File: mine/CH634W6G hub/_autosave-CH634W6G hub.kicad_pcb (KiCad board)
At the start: 2 copper layers, 5 parts, among them U1 CH634W6G, U2 *, U3 CH211D

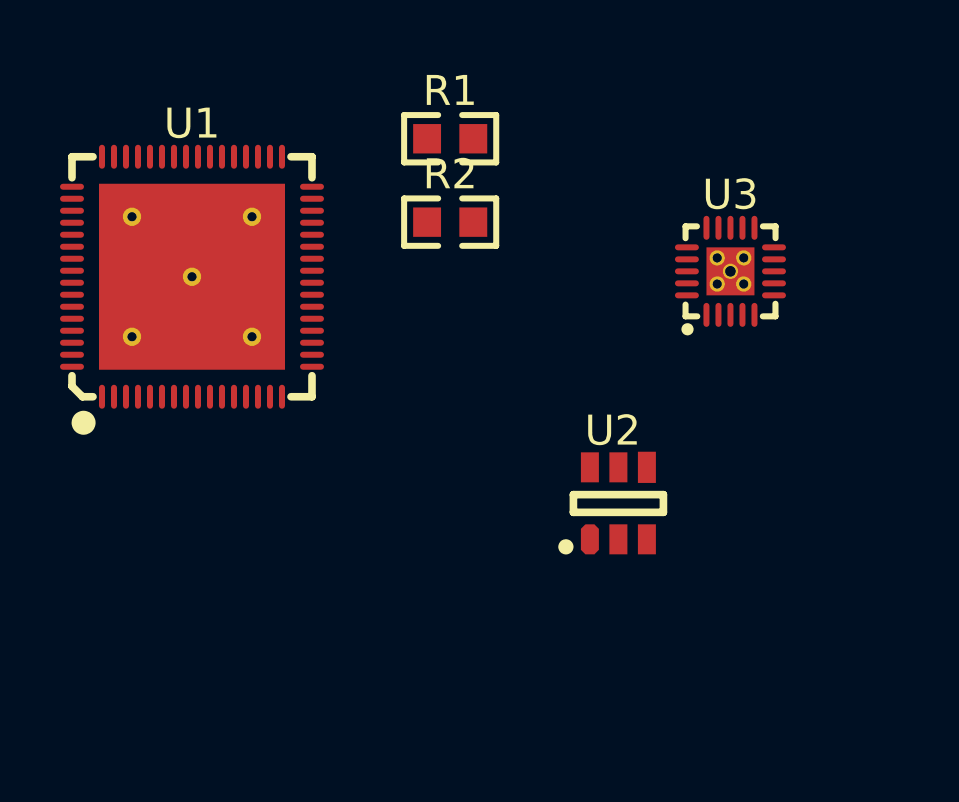
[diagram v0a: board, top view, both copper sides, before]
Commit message: why am I even redesigning the schematic, im just gonna use example, this is a backup
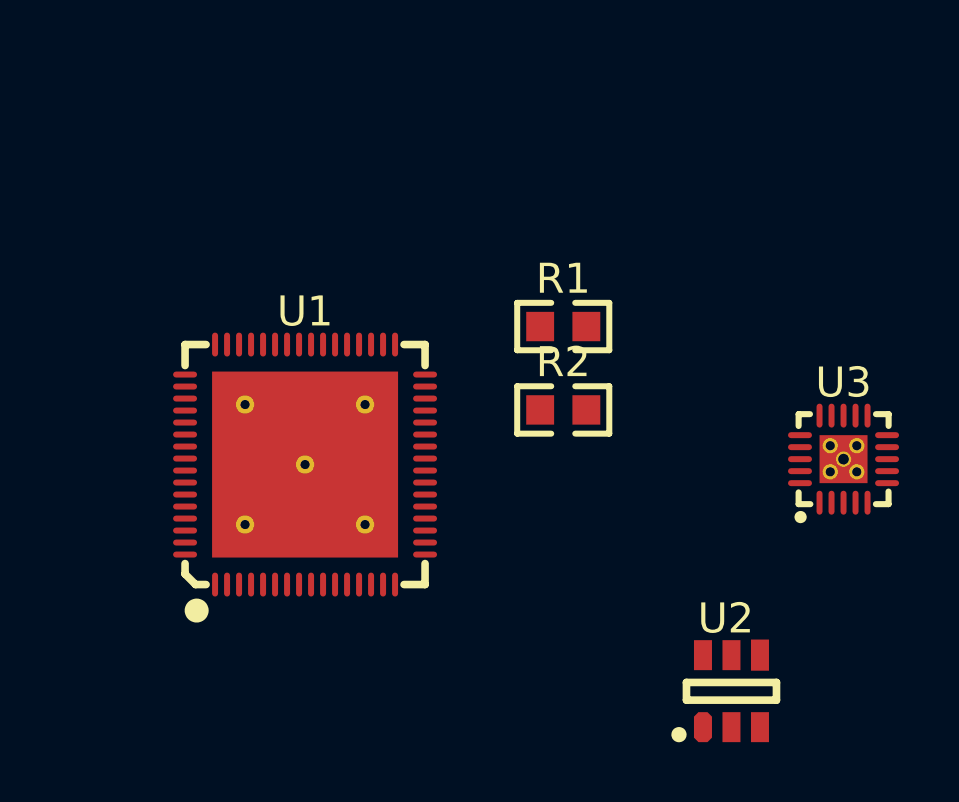
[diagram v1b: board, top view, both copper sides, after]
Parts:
- moved R1 7.31 mm to (113.0, 75.3)
- moved U1 7.31 mm to (105.1, 79.9)
- moved U2 7.31 mm to (118.4, 88.6)
- moved R2 7.31 mm to (113.0, 78.1)
- moved U3 7.31 mm to (123.1, 79.7)
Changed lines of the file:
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@@
 	(footprint "CHXXX:0603"
 		(layer "F.Cu")
-		(at 109.211 71.81)
+		(at 112.98 78.07)
 		(property "Reference" "R2"
 			(at 0.77 -1.59 0)
@@
 	(footprint "CHXXX:QFN20_3X3"
 		(layer "F.Cu")
-		(at 119.3238 73.45)
+		(at 123.0928 79.71)
 		(property "Reference" "U3"
 			(at 0 -2.5512 0)
@@
 	(footprint "CHXXX:0603"
 		(layer "F.Cu")
-		(at 109.211 69.03)
+		(at 112.98 75.29)
 		(property "Reference" "R1"
 			(at 0.77 -1.59 0)
@@
 	(footprint "CHXXX:QFN64_8X8"
 		(layer "F.Cu")
-		(at 101.375 73.63)
+		(at 105.144 79.89)
 		(property "Reference" "U1"
 			(at 0 -5.1 0)
@@
 	(footprint "CHXXX:SOT-23-6"
 		(layer "F.Cu")
-		(at 114.6385 82.383)
+		(at 118.4075 88.643)
 		(descr "SOT-23-6")
 		(property "Reference" "U2"
